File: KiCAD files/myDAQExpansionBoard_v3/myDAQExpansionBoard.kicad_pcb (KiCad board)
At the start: 2 copper layers, 100 x 100 mm, 61 parts, among them J1 OSTV7XX3151, J2 Conn_01x05_Male, J3 Conn_01x05_Male, J4 Screw_Terminal_01x02, J5 Screw_Terminal_01x01, J6 Screw_Terminal_01x02, J7 Conn_01x08_Male, J8 Screw_Terminal_01x01, SW1 SW_Push, SW2 SW_Push, SW3 SW_SPDT, SW4 SW_SPDT, U1 74LS47, U2 7segm-symbol, U3 ACS712xLCTR-05B, U4 LM35-D, U5 L293D

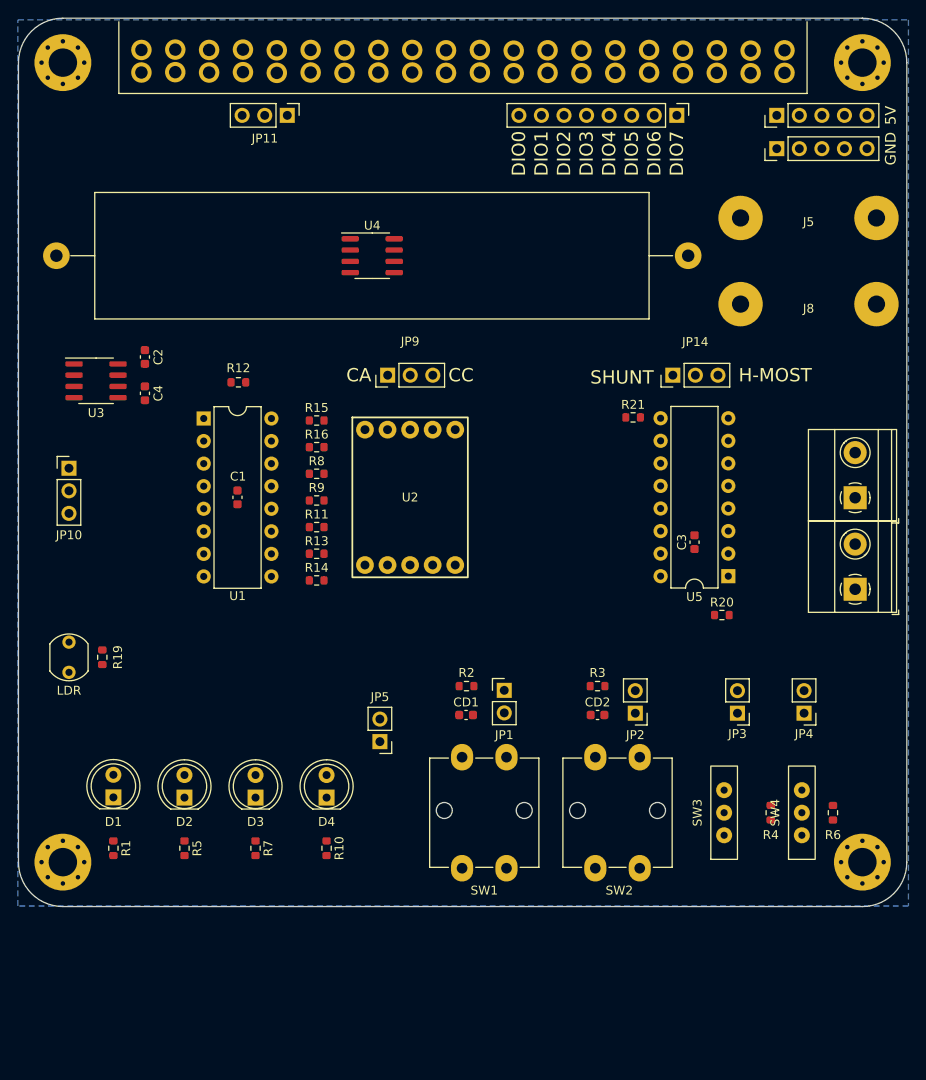
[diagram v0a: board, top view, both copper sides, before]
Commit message: update
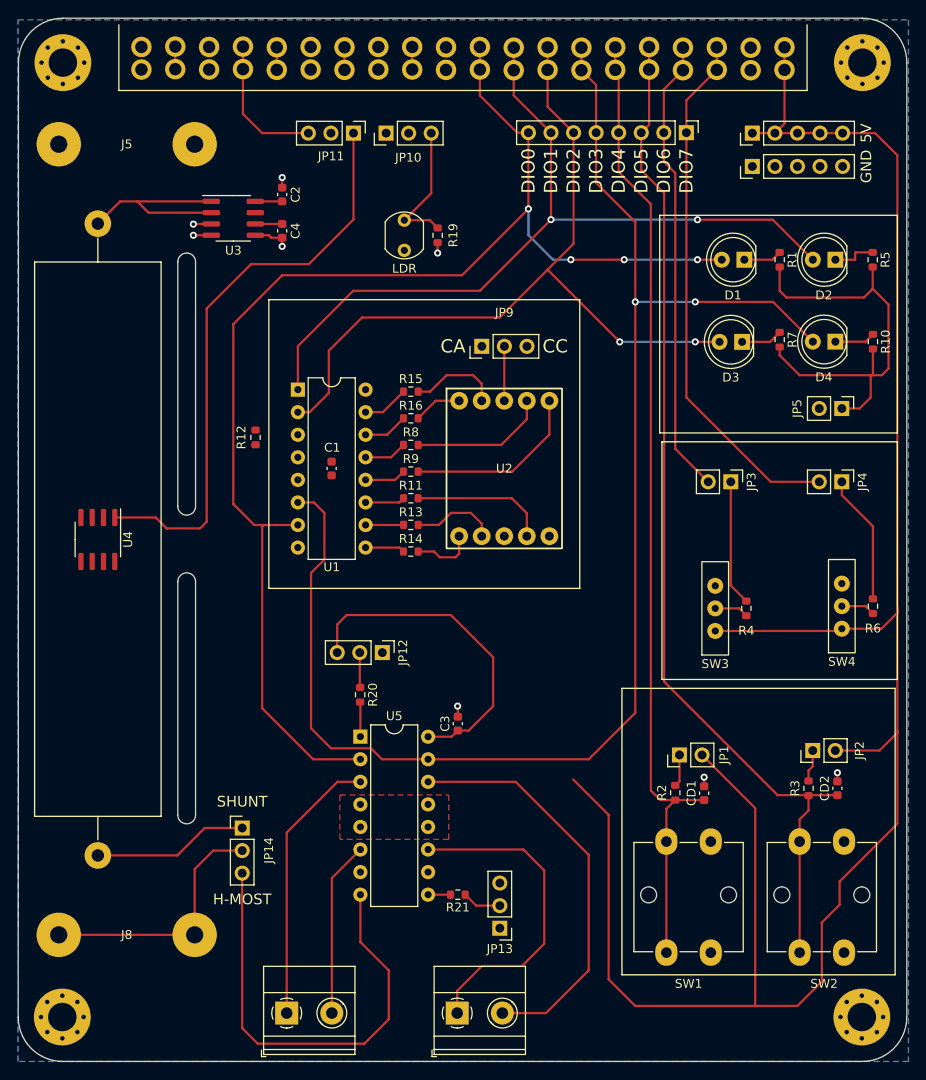
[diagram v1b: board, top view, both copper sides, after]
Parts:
- added JP12: Jumper_3_Open, Connector_PinHeader_2.54mm:PinHeader_1x03_P2.54mm_Vertical, F.Cu at (81.0, 117.0)
- added JP13: Jumper_3_Open, Connector_PinHeader_2.54mm:PinHeader_1x03_P2.54mm_Vertical, F.Cu at (94.2, 148.0)
- moved J8 104.6 mm to (52.2, 148.8), turned to 0 degrees
- moved R5 101.9 mm to (136.2, 72.8)
- moved R1 100.1 mm to (125.8, 72.8)
- moved D2 95.1 mm to (132.0, 72.8), turned to 180 degrees
- moved R17 94.7 mm to (49.0, 139.8), turned to 90 degrees
- moved D1 93.3 mm to (121.8, 72.8), turned to 180 degrees
- moved R10 83.9 mm to (136.2, 82.0)
- moved R7 82.2 mm to (125.8, 81.8)
- moved J4 79.8 mm to (70.3, 157.6), turned to 0 degrees
- moved J5 77.2 mm to (52.2, 59.8), turned to 0 degrees
- moved D4 76.9 mm to (132.0, 82.0), turned to 180 degrees
- moved D3 75.0 mm to (121.5, 82.0), turned to 180 degrees
- moved J6 73.3 mm to (89.5, 157.6), turned to 0 degrees
- moved JP14 70.3 mm to (65.2, 136.7), turned to 0 degrees
- moved JP5 64.1 mm to (132.8, 89.5), turned to -90 degrees
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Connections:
- R20 pad 1: +5V -> Net-(R20-Pad1)
- R21 pad 1: +5V -> Net-(R21-Pad1)
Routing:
- net +5V: track 0.00 -> 275.6 mm
- net DIO3: track 0.00 -> 167.7 mm, vias 0 -> 2
- net DIO0: track 0.00 -> 148.3 mm, vias 0 -> 4
- net DIO5: track 0.00 -> 115.8 mm
- net DIO4: track 0.00 -> 109.4 mm
- net DIO1: track 0.00 -> 91.7 mm, vias 0 -> 2
- net DIO2: track 0.00 -> 87.7 mm, vias 0 -> 2
- net Net-(JP11-Pad1): track 0.00 -> 65.6 mm
- net DIO7: track 0.00 -> 59.7 mm
- net DIO6: track 0.00 -> 51.8 mm
- net VDD: track 0.00 -> 51.2 mm
- net Net-(JP5-Pad1): track 0.00 -> 49.7 mm
- net Net-(J6-Pad2): track 0.00 -> 46.2 mm
- net Net-(J6-Pad1): track 0.00 -> 36.8 mm
- net Net-(J4-Pad1): track 0.00 -> 31.0 mm
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- added copper zone on F.Cu, net GND
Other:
- board size 100 x 100 mm -> 100 x 117.4 mm
